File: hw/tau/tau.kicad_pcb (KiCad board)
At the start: 2 copper layers, 100 x 70 mm, 50 parts, among them J1 USB_B, J2 AudioIn, J3 AudioOut, SW1 SW_bypass, SW2 SW_cahnnel_up, SW3 SW_midi, SW4 SW_sustain, SW5 SW_channel_down, U1 MCP6002-xMS

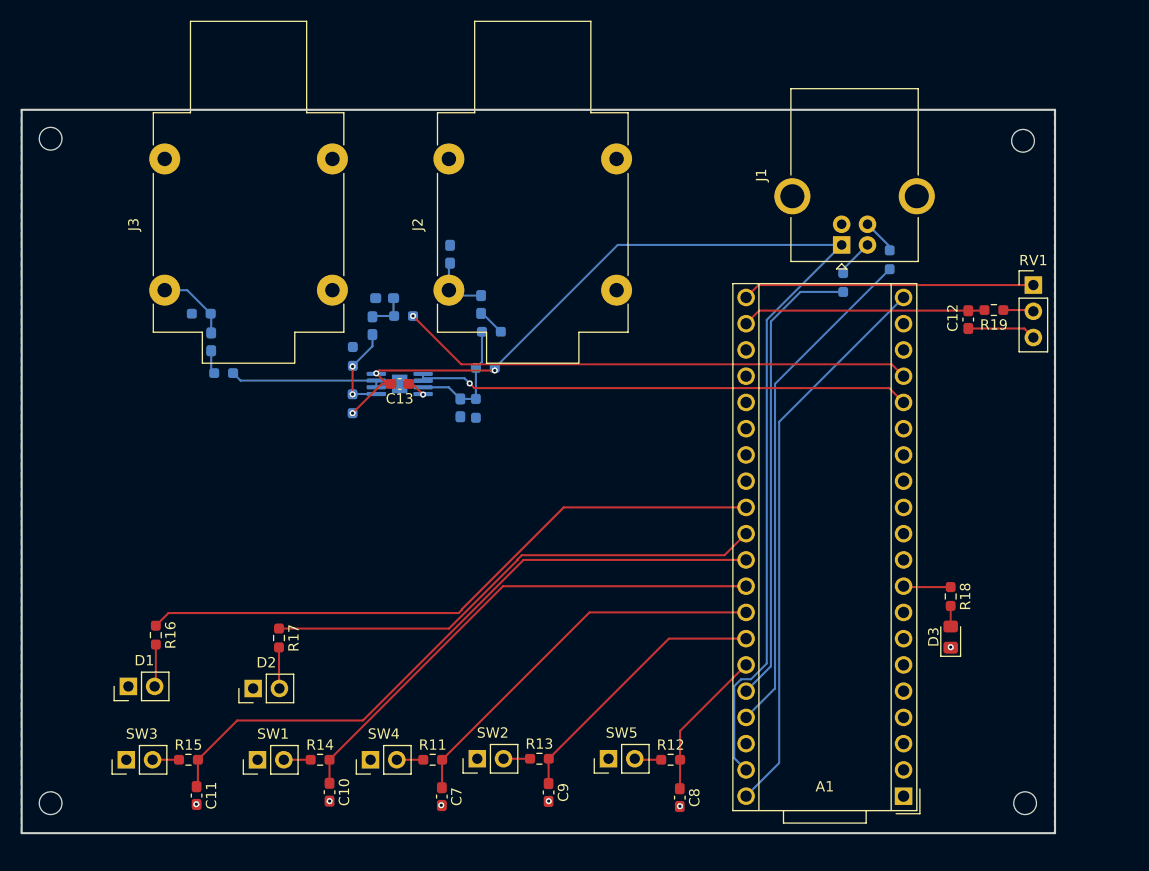
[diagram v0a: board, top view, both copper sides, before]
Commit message: god is dead and we killed him. new pcb.
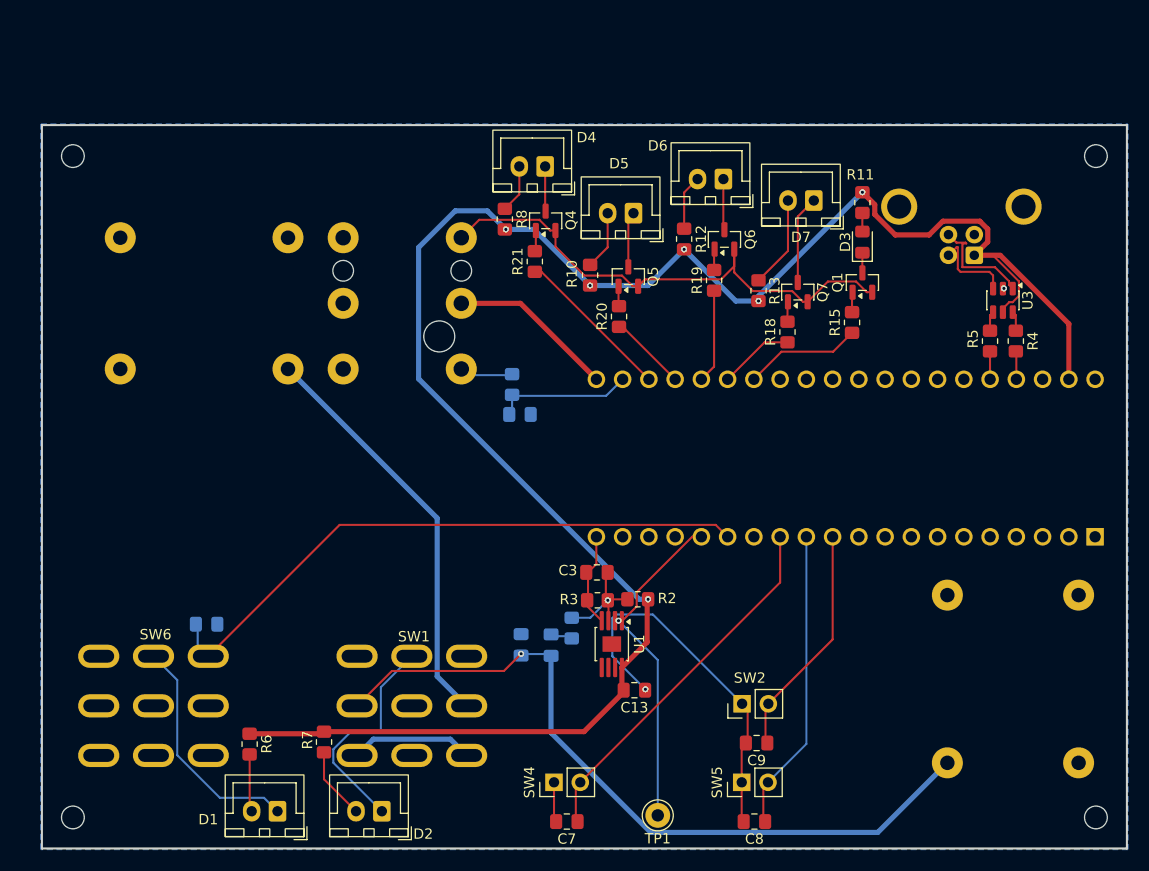
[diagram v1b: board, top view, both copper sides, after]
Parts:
- removed C10: 100n, Capacitor_SMD:C_0603_1608Metric_Pad1.08x0.95mm_HandSolder
- removed C4: 2n2, Capacitor_SMD:C_0603_1608Metric_Pad1.08x0.95mm_HandSolder
- removed C5, C6: 1u, Capacitor_SMD:C_0603_1608Metric_Pad1.08x0.95mm_HandSolder
- removed R16, R17: 68, Resistor_SMD:R_0603_1608Metric_Pad0.98x0.95mm_HandSolder
- removed R9: 1K, Resistor_SMD:R_0603_1608Metric_Pad0.98x0.95mm_HandSolder
- removed RV1: 50K, Connector_PinHeader_2.54mm:PinHeader_1x03_P2.54mm_Vertical
- removed SW3: SW_midi, Connector_PinHeader_2.54mm:PinHeader_1x02_P2.54mm_Vertical
- added D4: LED_channel1, Connector_JST:JST_XH_B2B-XH-A_1x02_P2.50mm_Vertical, F.Cu at (148.7, 64.0)
- added D5: LED_channel2, Connector_JST:JST_XH_B2B-XH-A_1x02_P2.50mm_Vertical, F.Cu at (157.2, 68.5)
- added D6: LED_channel3, Connector_JST:JST_XH_B2B-XH-A_1x02_P2.50mm_Vertical, F.Cu at (165.9, 65.2)
- added D7: LED_channel4, Connector_JST:JST_XH_B2B-XH-A_1x02_P2.50mm_Vertical, F.Cu at (174.7, 67.3)
- added J4: ExpressionTRS, Connector_Audio:Jack_6.35mm_Neutrik_NRJ6HH-AU_Horizontal, B.Cu at (140.6, 83.6)
- added Q1: 2N7002, Package_TO_SOT_SMD:SOT-23, F.Cu at (179.4, 75.2)
- added Q4: 2N7002, Package_TO_SOT_SMD:SOT-23, F.Cu at (148.8, 69.3)
- added Q5: 2N7002, Package_TO_SOT_SMD:SOT-23, F.Cu at (156.8, 74.7)
- added Q6: 2N7002, Package_TO_SOT_SMD:SOT-23, F.Cu at (166.1, 71.1)
- added Q7: 2N7002, Package_TO_SOT_SMD:SOT-23, F.Cu at (173.2, 76.2)
- added R20: 100, Resistor_SMD:R_0805_2012Metric_Pad1.20x1.40mm_HandSolder, F.Cu at (155.8, 78.5)
- added R21: 100, Resistor_SMD:R_0805_2012Metric_Pad1.20x1.40mm_HandSolder, F.Cu at (147.7, 73.2)
- added SW6: SW_3PDT_midi, 3pdt:SW_3PDT, F.Cu at (111.0, 110.0)
- added TP1: TestPoint, Connector_Pin:Pin_D1.0mm_L10.0mm_LooseFit, F.Cu at (159.6, 126.8)
- added U3: USBLC6-2SC6, Package_TO_SOT_SMD:SOT-23-6, F.Cu at (193.0, 77.0)
- A1, J1, J2, J3: moved to B.Cu
- C1: value 1u -> 10u; footprint Capacitor_SMD:C_0603_1608Metric_Pad1.08x0.95mm_HandSolder -> Capacitor_SMD:C_0805_2012Metric_Pad1.18x1.45mm_HandSolder
- C11, C12: footprint Capacitor_SMD:C_0603_1608Metric_Pad1.08x0.95mm_HandSolder -> Capacitor_SMD:C_0805_2012Metric_Pad1.18x1.45mm_HandSolder; moved to B.Cu
- C13, C2, C7, C8, C9: footprint Capacitor_SMD:C_0603_1608Metric_Pad1.08x0.95mm_HandSolder -> Capacitor_SMD:C_0805_2012Metric_Pad1.18x1.45mm_HandSolder
- C3: value 1n -> 10n; footprint Capacitor_SMD:C_0603_1608Metric_Pad1.08x0.95mm_HandSolder -> Capacitor_SMD:C_0805_2012Metric_Pad1.18x1.45mm_HandSolder; moved to F.Cu
- D1, D2: footprint Connector_PinHeader_2.54mm:PinHeader_1x02_P2.54mm_Vertical -> Connector_JST:JST_XH_B2B-XH-A_1x02_P2.50mm_Vertical
- R1: footprint Resistor_SMD:R_0603_1608Metric_Pad0.98x0.95mm_HandSolder -> Resistor_SMD:R_0805_2012Metric_Pad1.20x1.40mm_HandSolder
- R10, R8: value 1M -> 270; footprint Resistor_SMD:R_0603_1608Metric_Pad0.98x0.95mm_HandSolder -> Resistor_SMD:R_0805_2012Metric_Pad1.20x1.40mm_HandSolder; moved to F.Cu
- R11, R12, R13: value 10K -> 270; footprint Resistor_SMD:R_0603_1608Metric_Pad0.98x0.95mm_HandSolder -> Resistor_SMD:R_0805_2012Metric_Pad1.20x1.40mm_HandSolder
- R14: value 10K -> 1K; footprint Resistor_SMD:R_0603_1608Metric_Pad0.98x0.95mm_HandSolder -> Resistor_SMD:R_0805_2012Metric_Pad1.20x1.40mm_HandSolder; moved to B.Cu
- R15: value 10K -> 100; footprint Resistor_SMD:R_0603_1608Metric_Pad0.98x0.95mm_HandSolder -> Resistor_SMD:R_0805_2012Metric_Pad1.20x1.40mm_HandSolder
- R18: value 68 -> 100; footprint Resistor_SMD:R_0603_1608Metric_Pad0.98x0.95mm_HandSolder -> Resistor_SMD:R_0805_2012Metric_Pad1.20x1.40mm_HandSolder
- R19: value 1K -> 100; footprint Resistor_SMD:R_0603_1608Metric_Pad0.98x0.95mm_HandSolder -> Resistor_SMD:R_0805_2012Metric_Pad1.20x1.40mm_HandSolder
- R2, R3: value 1M -> 10K; footprint Resistor_SMD:R_0603_1608Metric_Pad0.98x0.95mm_HandSolder -> Resistor_SMD:R_0805_2012Metric_Pad1.20x1.40mm_HandSolder; moved to F.Cu
- R4, R5: footprint Resistor_SMD:R_0603_1608Metric_Pad0.98x0.95mm_HandSolder -> Resistor_SMD:R_0805_2012Metric_Pad1.20x1.40mm_HandSolder; moved to F.Cu
- R6: value 3K3 -> 270; footprint Resistor_SMD:R_0603_1608Metric_Pad0.98x0.95mm_HandSolder -> Resistor_SMD:R_0805_2012Metric_Pad1.20x1.40mm_HandSolder; moved to F.Cu
- R7: value 1K -> 270; footprint Resistor_SMD:R_0603_1608Metric_Pad0.98x0.95mm_HandSolder -> Resistor_SMD:R_0805_2012Metric_Pad1.20x1.40mm_HandSolder; moved to F.Cu
- SW1: value SW_bypass -> SW_3PDT_bypass; footprint Connector_PinHeader_2.54mm:PinHeader_1x02_P2.54mm_Vertical -> 3pdt:SW_3PDT
- SW2: value SW_cahnnel_up -> SW_channel_up
- U1: moved to F.Cu
- moved R15 76.9 mm to (178.4, 79.1), turned to 90 degrees
- moved R11 68.1 mm to (179.4, 67.5), turned to 90 degrees
- moved J2 66.5 mm to (187.6, 121.7), turned to 0 degrees
- moved R12 50.4 mm to (162.2, 71.0), turned to -90 degrees
- moved R13 50.0 mm to (169.3, 76.0), turned to -90 degrees
- moved C12 44.3 mm to (146.3, 88.0), turned to 0 degrees
- moved R6 44.0 mm to (120.1, 119.9), turned to -90 degrees
- moved R14 40.8 mm to (145.5, 85.1), turned to -90 degrees
- moved D3 39.2 mm to (179.4, 71.3)
- moved C2 38.4 mm to (146.4, 110.3)
- moved C13 37.3 mm to (157.3, 114.7)
- moved R7 37.0 mm to (127.3, 119.7), turned to -90 degrees
- moved C1 33.7 mm to (149.3, 110.3), turned to -90 degrees
- moved U1 32.5 mm to (155.2, 110.2), turned to -90 degrees
- moved A1 31.2 mm to (201.9, 99.8), turned to 90 degrees
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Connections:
- A1 pad 11: unconnected-(A1-SPI1_PICO-Pad11) -> channel_up_switch
- A1 pad 12: unconnected-(A1-I2C1_SCL-Pad12) -> channel_down_switch
- A1 pad 13: unconnected-(A1-I2C1_SDA-Pad13) -> sustain_switch
- A1 pad 15: unconnected-(A1-USART1_RX-Pad15) -> midi_switch
- A1 pad 17: audio_out -> unconnected-(A1-AUDIO_IN_2-Pad17)
- A1 pad 23: unconnected-(A1-ADC_1-Pad23) -> channel1_led
- A1 pad 24: unconnected-(A1-ADC_2-Pad24) -> channel2_led
- A1 pad 25: unconnected-(A1-ADC_3-Pad25) -> channel3_led
- A1 pad 26: unconnected-(A1-ADC_4-Pad26) -> channel4_led
- A1 pad 27: unconnected-(A1-ADC_5-Pad27) -> debug_led
- A1 pad 29: midi_led -> unconnected-(A1-DAC_OUT2-Pad29)
- A1 pad 30: bypass_led -> unconnected-(A1-DAC_OUT1-Pad30)
- A1 pad 31: midi_switch -> unconnected-(A1-SAI2_MCLK-Pad31)
- A1 pad 32: bypass_switch -> unconnected-(A1-SAI2_SD_B-Pad32)
- A1 pad 33: sustain_switch -> unconnected-(A1-SAI2_SD_A-Pad33)
- A1 pad 34: channel_up_switch -> unconnected-(A1-SAI2_FS-Pad34)
- A1 pad 35: channel_down_switch -> unconnected-(A1-SAI2_SCK-Pad35)
- A1 pad 9: debug_led -> unconnected-(A1-SPI1_SCK-Pad9)
- D1 pad 1: GND -> Net-(D1-K)
- D2 pad 1: GND -> Net-(D2-K)
- D3 pad 1: GND -> Net-(D3-K)
- J1 pad 2: Net-(J1-D-) -> /USB-D-
- J1 pad 3: Net-(J1-D+) -> /USB-D+
- J3 pad T: Net-(C6-Pad2) -> Net-(J3-PadT)
- R10 pad 1: Net-(U1B-+) -> Net-(D5-A)
- R10 pad 2: GND -> 5V
- R11 pad 1: Net-(SW4-B) -> Net-(D3-A)
- R11 pad 2: sustain_switch -> 5V
- R12 pad 1: Net-(SW5-B) -> Net-(D6-A)
- R12 pad 2: channel_down_switch -> 5V
- R13 pad 1: Net-(SW2-B) -> Net-(D7-A)
- R13 pad 2: channel_up_switch -> 5V
- R14 pad 1: Net-(SW1-B) -> Net-(J4-PadT)
- R14 pad 2: bypass_switch -> expression_pedal
- R15 pad 1: Net-(SW3-B) -> debug_led
- R15 pad 2: midi_switch -> Net-(Q1-G)
- R18 pad 1: debug_led -> channel4_led
- R18 pad 2: Net-(D3-A) -> Net-(Q7-G)
- R19 pad 1: Net-(R19-Pad1) -> channel3_led
- R19 pad 2: expression_pedal -> Net-(Q6-G)
- R4 pad 1: Net-(J1-D+) -> Net-(R4-Pad1)
- R5 pad 1: Net-(J1-D-) -> Net-(R5-Pad1)
- R6 pad 1: audio_out -> 5V
- R6 pad 2: Net-(C4-Pad1) -> Net-(D1-A)
- R7 pad 1: Net-(U1B--) -> 5V
- R7 pad 2: Net-(C6-Pad1) -> Net-(D2-A)
- R8 pad 1: 5V -> Net-(D4-A)
- R8 pad 2: Net-(U1B-+) -> 5V
- SW1 pad 1: GND -> unconnected-(SW1-Pad1)
- SW1 pad 2: Net-(SW1-B) -> Net-(C1-Pad2)
- SW2 pad 2: Net-(SW2-B) -> channel_up_switch
- SW4 pad 2: Net-(SW4-B) -> sustain_switch
- SW5 pad 2: Net-(SW5-B) -> channel_down_switch
- U1 pad 5: Net-(U1B-+) -> (no net)
- U1 pad 6: Net-(U1B--) -> (no net)
- U1 pad 7: Net-(U1B--) -> (no net)
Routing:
- net 5V: track 112.9 -> 192.3 mm, vias 3 -> 6
- net Net-(C1-Pad2): track 5.99 -> 73.5 mm, vias 0 -> 1
- net midi_led: track 61.9 -> 0.00 mm
- net audio_out: track 49.9 -> 0.00 mm, vias 1 -> 0
- net bypass_switch: track 49.5 -> 0.00 mm
- net bypass_led: track 49.0 -> 0.00 mm
- net Net-(A1-USB_D_+): track 49.1 -> 2.90 mm
- net Net-(A1-USB_D_-): track 44.9 -> 2.88 mm
- net Net-(J3-PadT): track 0.00 -> 39.8 mm
- net GND: track 63.3 -> 100.9 mm, vias 7 -> 2
- net Net-(D1-K): track 0.00 -> 22.5 mm
- net Net-(D2-K): track 0.00 -> 21.8 mm
- net channel1_led: track 0.00 -> 15.3 mm
- net audio_in: track 48.1 -> 33.3 mm
- net Net-(U1B--): track 14.8 -> 0.00 mm
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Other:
- board size 100 x 70 mm -> 105 x 70 mm
